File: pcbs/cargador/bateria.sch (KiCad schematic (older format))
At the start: 17 parts, among them U1 BQ24004

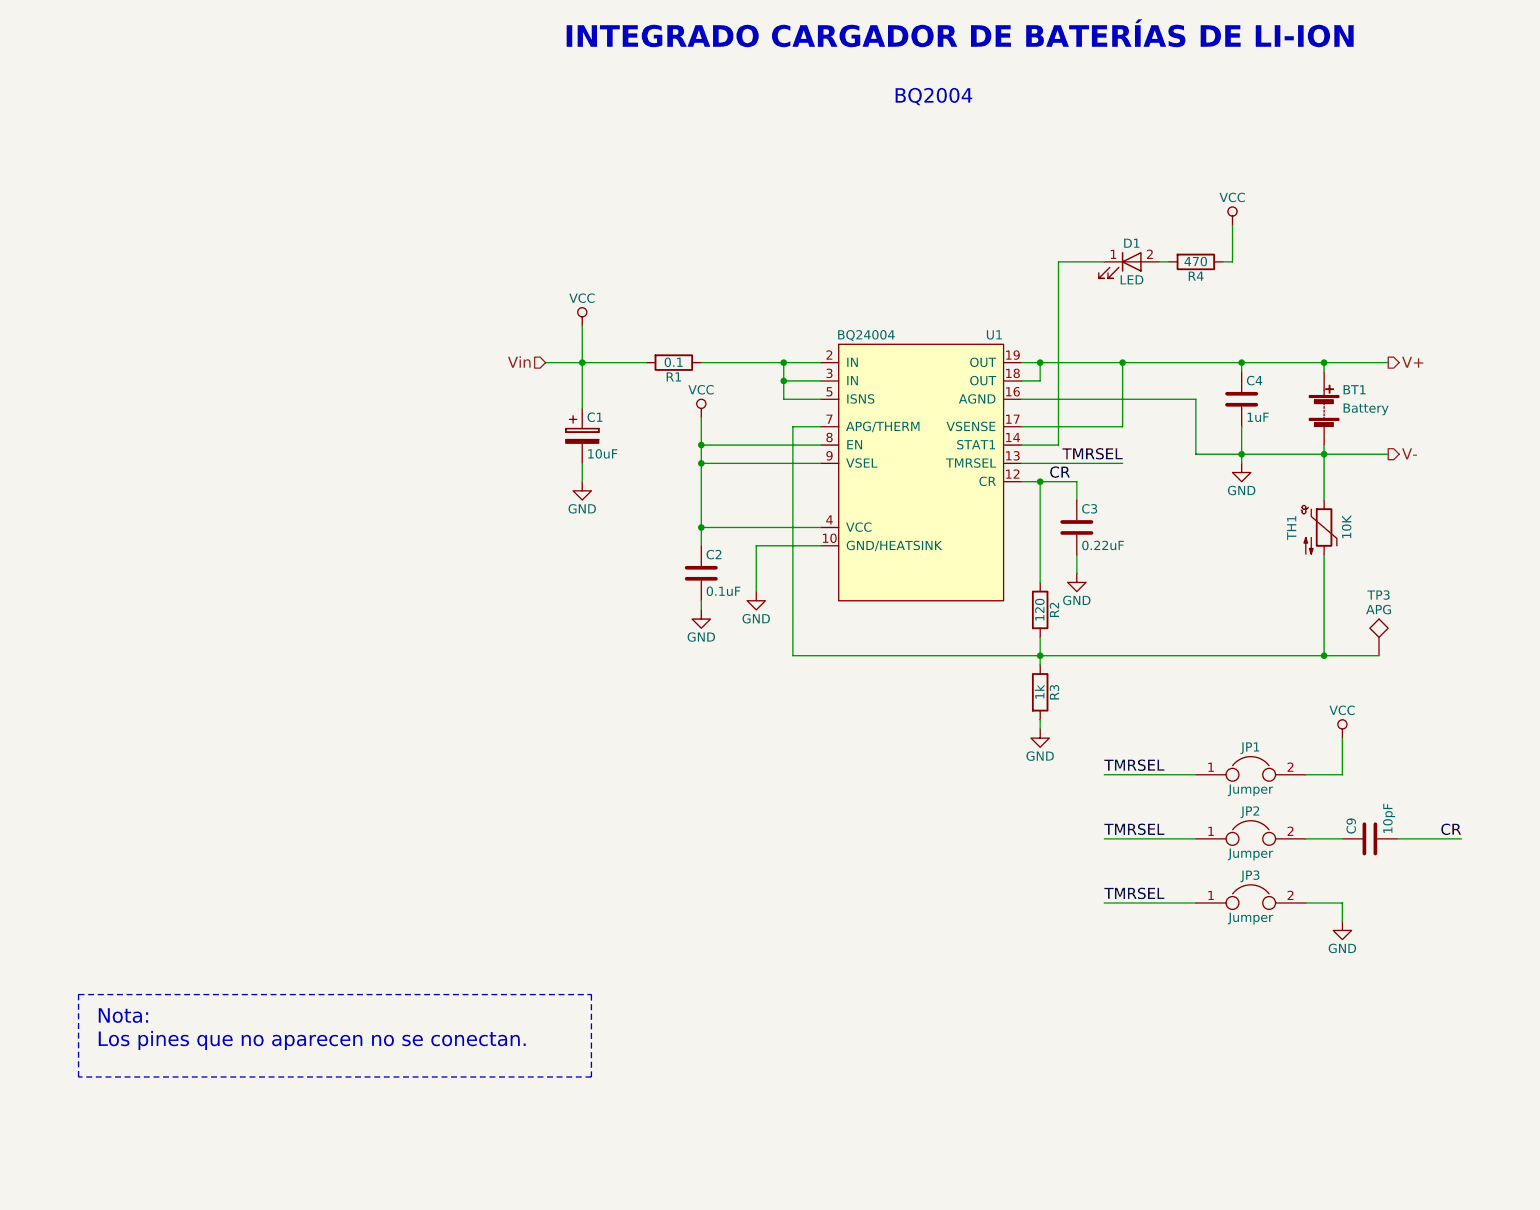
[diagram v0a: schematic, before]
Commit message: correcciones en los pdfs de los pcb
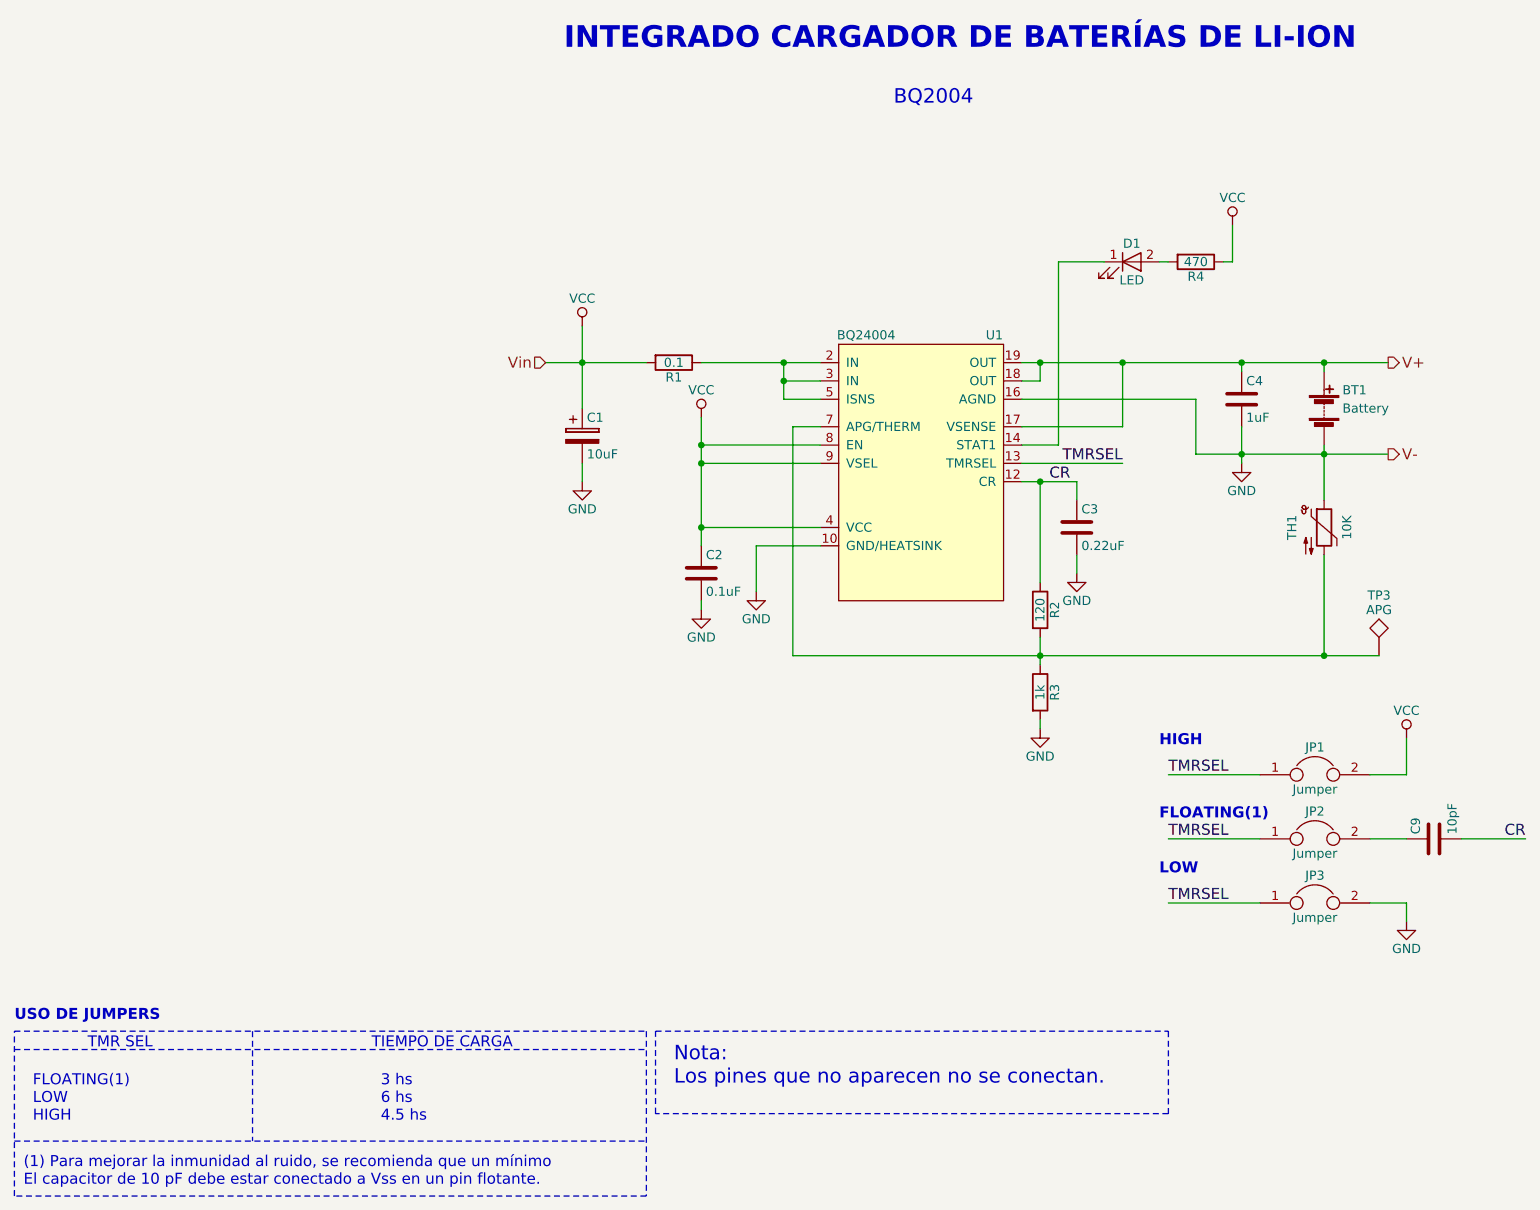
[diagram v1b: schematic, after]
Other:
- note added: "(1) Para mejorar la inmunidad al ruido, se recomienda que un mínimo\nEl capacitor de 10 pF debe estar conectado a Vss en un pin flotante."
- note added: "3 hs\n6 hs\n4.5 hs"
- note added: "FLOATING(1)"
- note added: "FLOATING(1)\nLOW\nHIGH"
- note added: "HIGH"
- note added: "LOW"
- note added: "TIEMPO DE CARGA"
- note added: "TMR SEL"
- note added: "USO DE JUMPERS"
- moved on the sheet: C9, JP1, JP2, JP3
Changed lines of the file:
@@
 	1    0    0    -1
 $EndComp
-Wire Wire Line
-	3650 2800 3650 3250
-Wire Wire Line
-	3450 3000 4000 3000
-Connection ~ 3650 3000
-Wire Wire Line
-	3650 3550 3650 3650
-Wire Wire Line
-	4300 3000 4950 3000
-Wire Wire Line
-	4750 3000 4750 3200
-Wire Wire Line
-	4750 3100 4950 3100
-Connection ~ 4750 3000
-Wire Wire Line
-	4750 3200 4950 3200
-Connection ~ 4750 3100
-Wire Wire Line
-	4300 3450 4950 3450
-Connection ~ 4300 3450
-Wire Wire Line
-	4300 3550 4950 3550
-Connection ~ 4300 3550
-Wire Wire Line
-	4300 3900 4950 3900
-Connection ~ 4300 3900
-Wire Wire Line
-	4950 4000 4600 4000
-Wire Wire Line
-	4600 4000 4600 4250
-Wire Wire Line
-	4300 3300 4300 4000
-Wire Wire Line
-	4300 4300 4300 4350
-Wire Wire Line
-	4950 3350 4800 3350
-Wire Wire Line
-	6150 3650 6150 4200
 $Comp
 L R R2
@@
 	1    0    0    -1
 $EndComp
-Wire Wire Line
-	6150 5000 6150 4950
-Wire Wire Line
-	6150 4500 6150 4650
-Wire Wire Line
-	4800 4600 8000 4600
-Connection ~ 6150 4600
-Wire Wire Line
-	4800 3350 4800 4600
-Wire Wire Line
-	6350 3650 6350 3750
-Connection ~ 6150 3650
-Wire Wire Line
-	6350 4150 6350 4050
 $Comp
 L VCC #PWR015
 U 1 1 5B91CE4A
-P 7800 5050
-F 0 "#PWR015" H 7800 4900 50  0001 C CNN
-F 1 "VCC" H 7800 5200 50  0000 C CNN
-F 2 "" H 7800 5050 50  0001 C CNN
-F 3 "" H 7800 5050 50  0001 C CNN
-	1    7800 5050
-	1    0    0    -1
-$EndComp
-Wire Wire Line
-	6250 3450 6050 3450
-Wire Wire Line
-	6250 2450 6250 3450
+P 8150 5050
+F 0 "#PWR015" H 8150 4900 50  0001 C CNN
+F 1 "VCC" H 8150 5200 50  0000 C CNN
+F 2 "" H 8150 5050 50  0001 C CNN
+F 3 "" H 8150 5050 50  0001 C CNN
+	1    8150 5050
+	1    0    0    -1
+$EndComp
 $Comp
 L LED D1
@@
 	1    0    0    -1
 $EndComp
-Wire Wire Line
-	6250 2450 6500 2450
-Wire Wire Line
-	6800 2450 6850 2450
 $Comp
 L R R4
@@
 	0    1    1    0
 $EndComp
-Wire Wire Line
-	7150 2450 7200 2450
-Wire Wire Line
-	7200 2450 7200 2250
-Wire Wire Line
-	6050 3000 8050 3000
-Wire Wire Line
-	6150 3100 6150 3000
-Connection ~ 6150 3000
-Wire Wire Line
-	6050 3350 6600 3350
-Wire Wire Line
-	6600 3350 6600 3000
-Connection ~ 6600 3000
-Wire Wire Line
-	6050 3200 7000 3200
-Wire Wire Line
-	7000 3200 7000 3500
-Wire Wire Line
-	7250 3050 7250 3000
-Connection ~ 7250 3000
-Wire Wire Line
-	7000 3500 8050 3500
-Wire Wire Line
-	7250 3350 7250 3550
-Connection ~ 7250 3500
 $Comp
 L Battery BT1
@@
 	1    0    0    -1
 $EndComp
-Wire Wire Line
-	7700 3000 7700 3050
-Wire Wire Line
-	7700 3450 7700 3750
 $Comp
 L GND #PWR016
@@
 	1    0    0    -1
 $EndComp
-Connection ~ 7700 3500
 $Comp
 L Thermistor_NTC TH1
@@
 	1    0    0    -1
 $EndComp
-Wire Wire Line
-	7700 4600 7700 4050
-Connection ~ 7700 3000
 Text HLabel 8050 3500 2    60   Output ~ 0
 V-
@@
 	1    0    0    -1
 $EndComp
-Connection ~ 7700 4600
 $Comp
 L TEST TP3
@@
 	1    0    0    -1
 $EndComp
-Wire Wire Line
-	6050 3100 6150 3100
-Wire Wire Line
-	6050 3650 6350 3650
 $Comp
 L GND #PWR017
 U 1 1 5BA00C1E
-P 7800 6050
-F 0 "#PWR017" H 7800 5800 50  0001 C CNN
-F 1 "GND" H 7800 5900 50  0000 C CNN
-F 2 "" H 7800 6050 50  0001 C CNN
-F 3 "" H 7800 6050 50  0001 C CNN
-	1    7800 6050
+P 8150 6050
+F 0 "#PWR017" H 8150 5800 50  0001 C CNN
+F 1 "GND" H 8150 5900 50  0000 C CNN
+F 2 "" H 8150 6050 50  0001 C CNN
+F 3 "" H 8150 6050 50  0001 C CNN
+	1    8150 6050
 	1    0    0    -1
 $EndComp
@@
 L Jumper JP1
 U 1 1 5BA00EC7
-P 7300 5250
-F 0 "JP1" H 7300 5400 50  0000 C CNN
-F 1 "Jumper" H 7300 5170 50  0000 C CNN
-F 2 "Pin_Headers:Pin_Header_Straight_1x02_Pitch2.54mm" H 7300 5250 50  0001 C CNN
-F 3 "" H 7300 5250 50  0001 C CNN
-	1    7300 5250
+P 7650 5250
+F 0 "JP1" H 7650 5400 50  0000 C CNN
+F 1 "Jumper" H 7650 5170 50  0000 C CNN
+F 2 "Pin_Headers:Pin_Header_Straight_1x02_Pitch2.54mm" H 7650 5250 50  0001 C CNN
+F 3 "" H 7650 5250 50  0001 C CNN
+	1    7650 5250
 	1    0    0    -1
 $EndComp
@@
 L Jumper JP2
 U 1 1 5BA00FCC
-P 7300 5600
-F 0 "JP2" H 7300 5750 50  0000 C CNN
-F 1 "Jumper" H 7300 5520 50  0000 C CNN
-F 2 "Pin_Headers:Pin_Header_Straight_1x02_Pitch2.54mm" H 7300 5600 50  0001 C CNN
-F 3 "" H 7300 5600 50  0001 C CNN
-	1    7300 5600
+P 7650 5600
+F 0 "JP2" H 7650 5750 50  0000 C CNN
+F 1 "Jumper" H 7650 5520 50  0000 C CNN
+F 2 "Pin_Headers:Pin_Header_Straight_1x02_Pitch2.54mm" H 7650 5600 50  0001 C CNN
+F 3 "" H 7650 5600 50  0001 C CNN
+	1    7650 5600
 	1    0    0    -1
 $EndComp
@@
 L Jumper JP3
 U 1 1 5BA01026
-P 7300 5950
-F 0 "JP3" H 7300 6100 50  0000 C CNN
-F 1 "Jumper" H 7300 5870 50  0000 C CNN
-F 2 "Pin_Headers:Pin_Header_Straight_1x02_Pitch2.54mm" H 7300 5950 50  0001 C CNN
-F 3 "" H 7300 5950 50  0001 C CNN
-	1    7300 5950
-	1    0    0    -1
-$EndComp
-Wire Wire Line
-	6050 3550 6600 3550
+P 7650 5950
+F 0 "JP3" H 7650 6100 50  0000 C CNN
+F 1 "Jumper" H 7650 5870 50  0000 C CNN
+F 2 "Pin_Headers:Pin_Header_Straight_1x02_Pitch2.54mm" H 7650 5950 50  0001 C CNN
+F 3 "" H 7650 5950 50  0001 C CNN
+	1    7650 5950
+	1    0    0    -1
+$EndComp
 Text Label 6600 3550 2    60   ~ 0
 TMRSEL
-Text Label 6500 5250 0    60   ~ 0
+Text Label 6850 5250 0    60   ~ 0
 TMRSEL
-Text Label 6500 5600 0    60   ~ 0
+Text Label 6850 5600 0    60   ~ 0
 TMRSEL
-Text Label 6500 5950 0    60   ~ 0
+Text Label 6850 5950 0    60   ~ 0
 TMRSEL
-Wire Wire Line
-	7000 5250 6500 5250
-Wire Wire Line
-	7000 5600 6500 5600
-Wire Wire Line
-	7000 5950 6500 5950
-Wire Wire Line
-	7600 5250 7800 5250
-Wire Wire Line
-	7800 5250 7800 5050
-Wire Wire Line
-	7600 5600 7800 5600
-Wire Wire Line
-	7600 5950 7800 5950
-Wire Wire Line
-	7800 5950 7800 6050
-Text Label 8450 5600 2    60   ~ 0
+Text Label 8800 5600 2    60   ~ 0
 CR
 $Comp
 L C C9
 U 1 1 5BA01AAE
-P 7950 5600
-F 0 "C9" H 7975 5700 50  0000 L CNN
-F 1 "10pF" H 7975 5500 50  0000 L CNN
-F 2 "Capacitors_SMD:C_0805_HandSoldering" H 7988 5450 50  0001 C CNN
-F 3 "" H 7950 5600 50  0001 C CNN
-	1    7950 5600
+P 8300 5600
+F 0 "C9" H 8325 5700 50  0000 L CNN
+F 1 "10pF" H 8325 5500 50  0000 L CNN
+F 2 "Capacitors_SMD:C_0805_HandSoldering" H 8338 5450 50  0001 C CNN
+F 3 "" H 8300 5600 50  0001 C CNN
+	1    8300 5600
 	0    -1   -1   0
 $EndComp
-Wire Wire Line
-	8100 5600 8450 5600
 Text Notes 3550 1300 0    118  ~ 24
 INTEGRADO CARGADOR DE BATERÍAS DE LI-ION
 Text Notes 5350 1600 0    79   ~ 0
 BQ2004
-Text Notes 1000 6750 0    79   ~ 0
+Text Notes 4150 6950 0    79   ~ 0
 Nota:\nLos pines que no aparecen no se conectan.
-Wire Notes Line
-	900  6450 3700 6450
-Wire Notes Line
-	3700 6450 3700 6900
-Wire Notes Line
-	3700 6900 900  6900
-Wire Notes Line
-	900  6900 900  6450
+Text Notes 650  7150 0    60   ~ 0
+FLOATING(1)\nLOW\nHIGH
+Text Notes 2550 7150 0    60   ~ 0
+3 hs\n6 hs\n4.5 hs
+Text Notes 950  6750 0    60   ~ 0
+TMR SEL
+Text Notes 2500 6750 0    60   ~ 0
+TIEMPO DE CARGA
+Text Notes 600  7500 0    60   ~ 0
+(1) Para mejorar la inmunidad al ruido, se recomienda que un mínimo\nEl capacitor de 10 pF debe estar conectado a Vss en un pin flotante.
+Text Notes 550  6600 0    60   ~ 12
+USO DE JUMPERS
+Text Notes 6800 5100 0    60   ~ 12
+HIGH
+Text Notes 6800 5500 0    60   ~ 12
+FLOATING(1)
+Text Notes 6800 5800 0    60   ~ 12
+LOW
+Wire Wire Line
+	3650 2800 3650 3250
+Wire Wire Line
+	3450 3000 4000 3000
+Connection ~ 3650 3000
+Wire Wire Line
+	3650 3550 3650 3650
+Wire Wire Line
+	4300 3000 4950 3000
+Wire Wire Line
+	4750 3000 4750 3200
+Wire Wire Line
+	4750 3100 4950 3100
+Connection ~ 4750 3000
+Wire Wire Line
+	4750 3200 4950 3200
+Connection ~ 4750 3100
+Wire Wire Line
+	4300 3450 4950 3450
+Connection ~ 4300 3450
+Wire Wire Line
+	4300 3550 4950 3550
+Connection ~ 4300 3550
+Wire Wire Line
+	4300 3900 4950 3900
+Connection ~ 4300 3900
+Wire Wire Line
+	4950 4000 4600 4000
+Wire Wire Line
+	4600 4000 4600 4250
+Wire Wire Line
+	4300 3300 4300 4000
+Wire Wire Line
+	4300 4300 4300 4350
+Wire Wire Line
+	4950 3350 4800 3350
+Wire Wire Line
+	6150 3650 6150 4200
+Wire Wire Line
+	6150 5000 6150 4950
+Wire Wire Line
+	6150 4500 6150 4650
+Wire Wire Line
+	4800 4600 8000 4600
+Connection ~ 6150 4600
+Wire Wire Line
+	4800 3350 4800 4600
+Wire Wire Line
+	6350 3650 6350 3750
+Connection ~ 6150 3650
+Wire Wire Line
+	6350 4150 6350 4050
+Wire Wire Line
+	6250 3450 6050 3450
+Wire Wire Line
+	6250 2450 6250 3450
+Wire Wire Line
+	6250 2450 6500 2450
+Wire Wire Line
+	6800 2450 6850 2450
+Wire Wire Line
+	7150 2450 7200 2450
+Wire Wire Line
+	7200 2450 7200 2250
+Wire Wire Line
+	6050 3000 8050 3000
+Wire Wire Line
+	6150 3100 6150 3000
+Connection ~ 6150 3000
+Wire Wire Line
+	6050 3350 6600 3350
+Wire Wire Line
+	6600 3350 6600 3000
+Connection ~ 6600 3000
+Wire Wire Line
+	6050 3200 7000 3200
+Wire Wire Line
+	7000 3200 7000 3500
+Wire Wire Line
+	7250 3050 7250 3000
+Connection ~ 7250 3000
+Wire Wire Line
+	7000 3500 8050 3500
+Wire Wire Line
+	7250 3350 7250 3550
+Connection ~ 7250 3500
+Wire Wire Line
+	7700 3000 7700 3050
+Wire Wire Line
+	7700 3450 7700 3750
+Connection ~ 7700 3500
+Wire Wire Line
+	7700 4600 7700 4050
+Connection ~ 7700 3000
+Connection ~ 7700 4600
+Wire Wire Line
+	6050 3100 6150 3100
+Wire Wire Line
+	6050 3650 6350 3650
+Wire Wire Line
+	6050 3550 6600 3550
+Wire Wire Line
+	7350 5250 6850 5250
+Wire Wire Line
+	7350 5600 6850 5600
+Wire Wire Line
+	7350 5950 6850 5950
+Wire Wire Line
+	7950 5250 8150 5250
+Wire Wire Line
+	8150 5250 8150 5050
+Wire Wire Line
+	7950 5600 8150 5600
+Wire Wire Line
+	7950 5950 8150 5950
+Wire Wire Line
+	8150 5950 8150 6050
+Wire Wire Line
+	8450 5600 8800 5600
+Wire Notes Line
+	4050 6650 6850 6650
+Wire Notes Line
+	6850 6650 6850 7100
+Wire Notes Line
+	6850 7100 4050 7100
+Wire Notes Line
+	4050 7100 4050 6650
+Wire Notes Line
+	550  6650 4000 6650
+Wire Notes Line
+	4000 6650 4000 7550
+Wire Notes Line
+	4000 7550 550  7550
+Wire Notes Line
+	550  7550 550  6650
+Wire Notes Line
+	550  6750 4000 6750
+Wire Notes Line
+	550  7250 4000 7250
+Wire Notes Line
+	1850 6650 1850 7250
 $EndSCHEMATC
